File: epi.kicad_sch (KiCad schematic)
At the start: 29 parts, among them J1 Connector 1x12, J2 Connector 1x12, J3 Conn_01x05, J4 USB-C 2.0 mid-mount female co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, U1 ATmega32U4-M, Y1 Crystal_GND24_Small

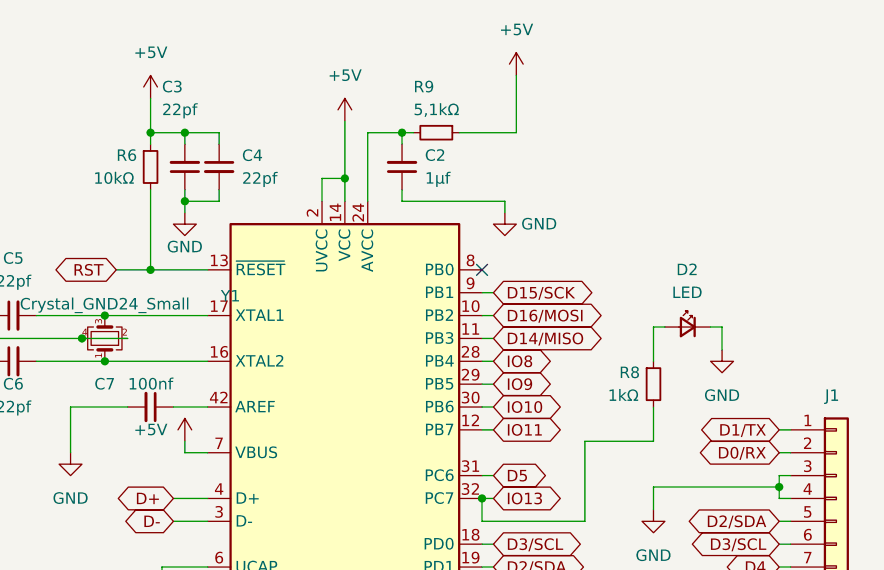
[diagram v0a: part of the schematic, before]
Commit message: fail
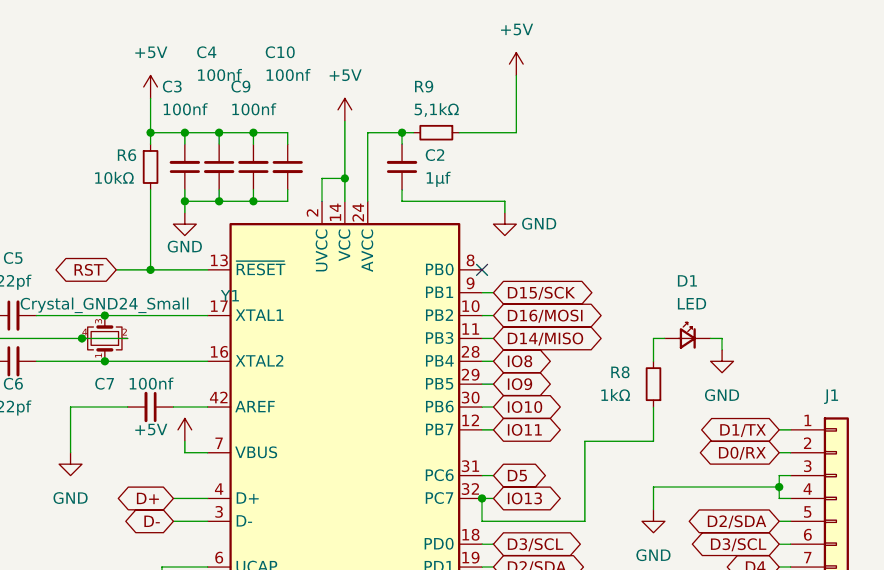
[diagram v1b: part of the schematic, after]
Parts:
- added C10, C9: 100nf, Capacitor_SMD:C_0402_1005Metric, symbol Device:C_Small
- C3, C4: value 22pf -> 100nf
- renumbered D2 to D1
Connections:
- net +5V: now also C10.1, C9.2
- net GND: now also C10.2, C9.1
- net IO13: now also R8.1; no longer R8.2
- net at D1.2 (A): now also R8.2; no longer R8.1
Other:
- moved on the sheet: D1, R8
